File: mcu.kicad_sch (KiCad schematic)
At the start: 15 parts, among them SW1 RST, SW2 BOOT, U1 ESP32-S3-WROOM-1

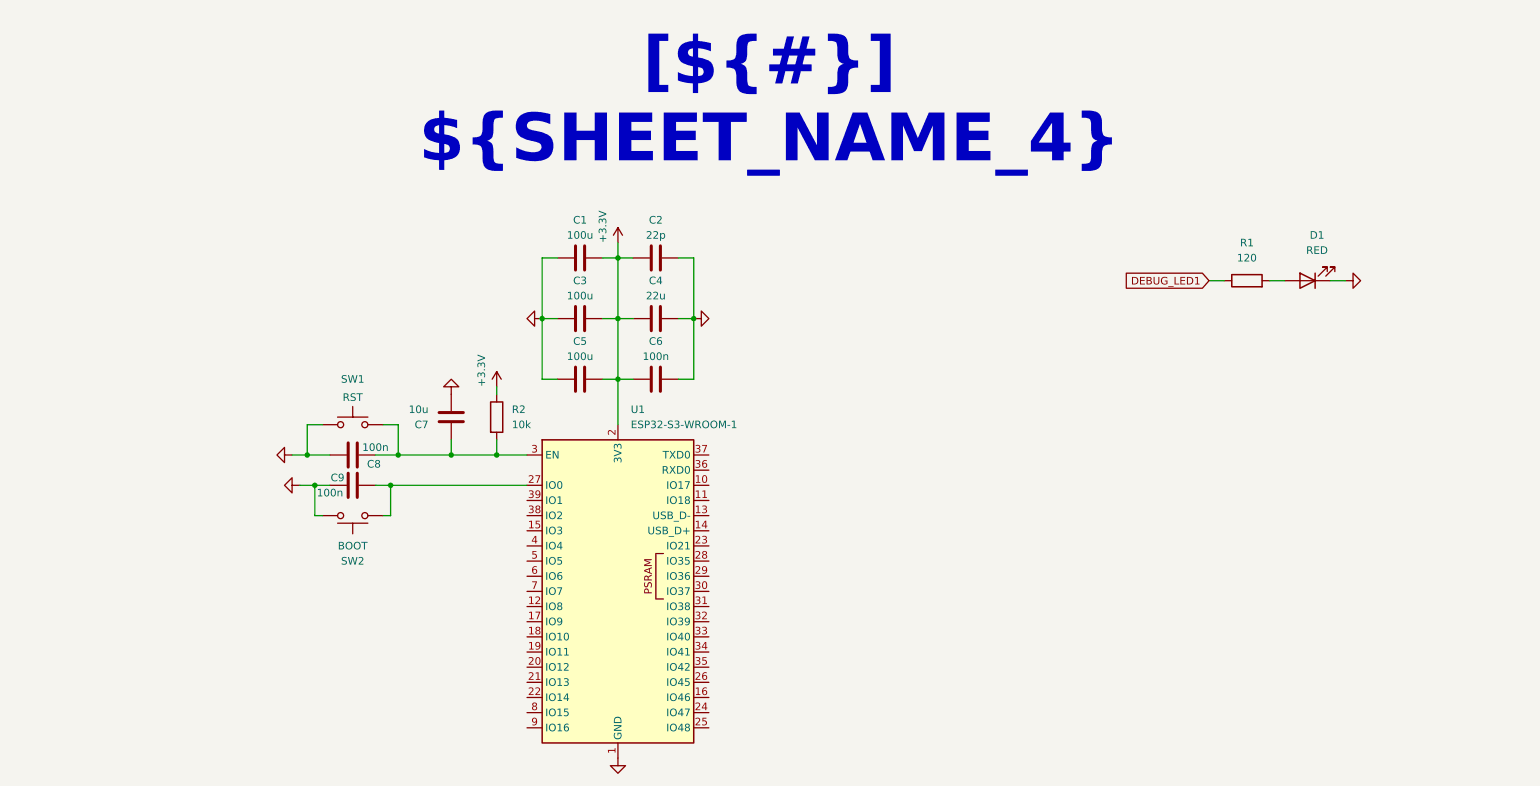
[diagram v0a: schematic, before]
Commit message: PCB schematic design
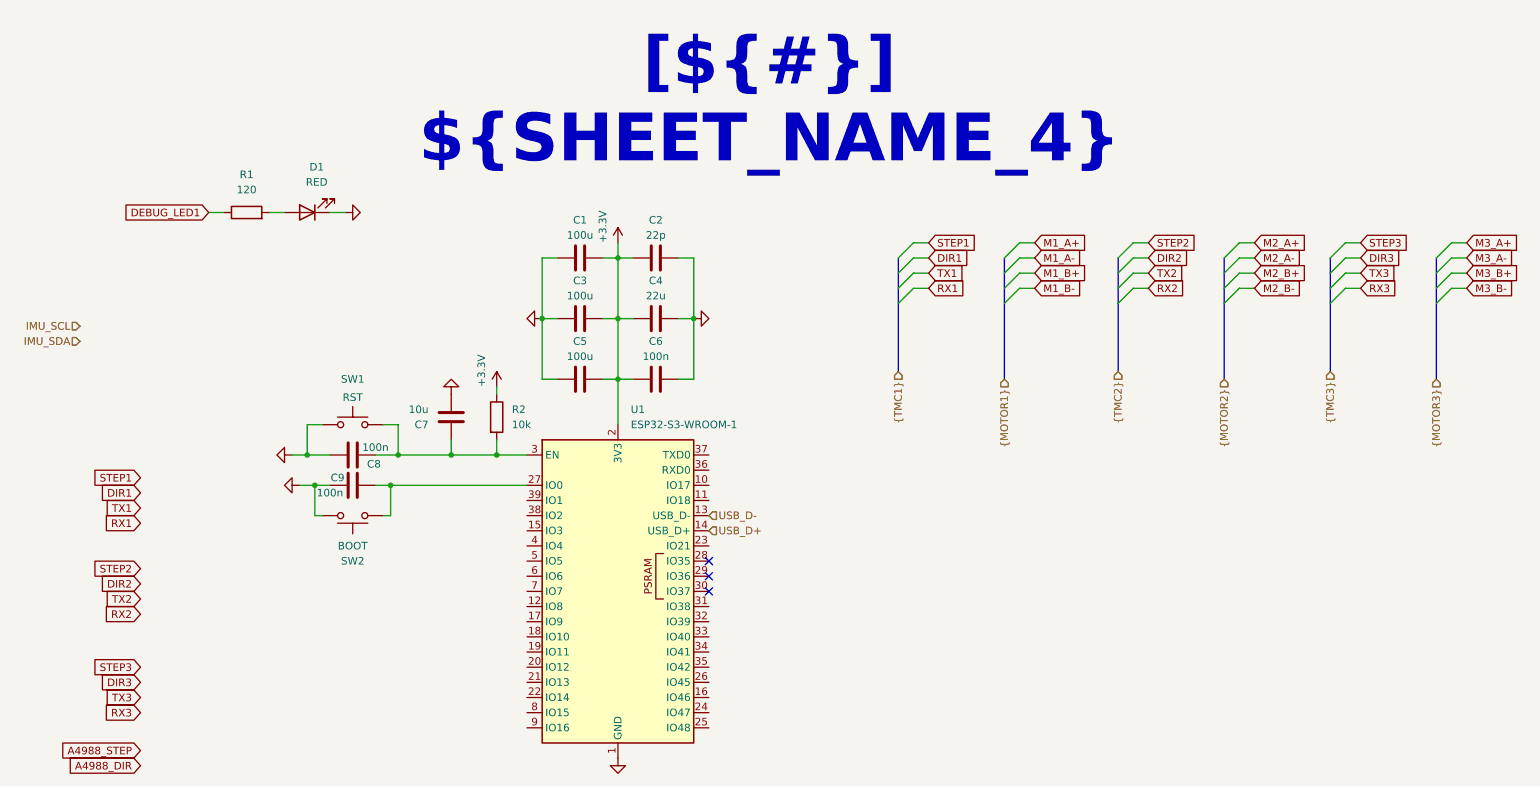
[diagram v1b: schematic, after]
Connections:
- net USB_D-: now reaches U1.13 (USB_D-)
- net USB_D+: now reaches U1.14 (USB_D+)
- no-connect marks 0 -> 3
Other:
- moved on the sheet: D1, R1
